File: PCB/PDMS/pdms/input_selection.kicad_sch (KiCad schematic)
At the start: 31 parts, among them U1 AQY221R4VY, U4 AQY221R4VY, U5 AQY221R4VY, U6 AQY221R4VY

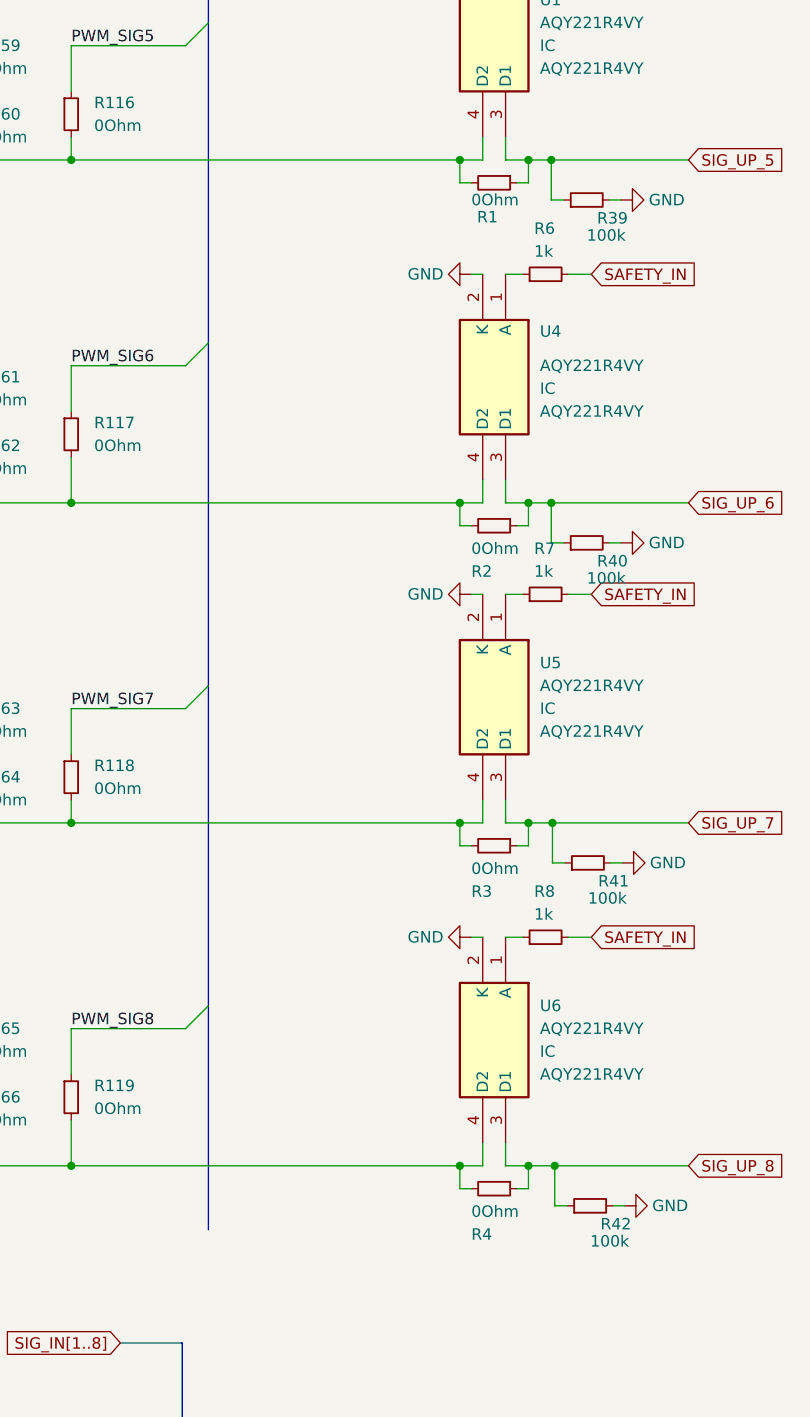
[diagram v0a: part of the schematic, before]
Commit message: Minor changes in overall schematics & MP4322 scheamtics
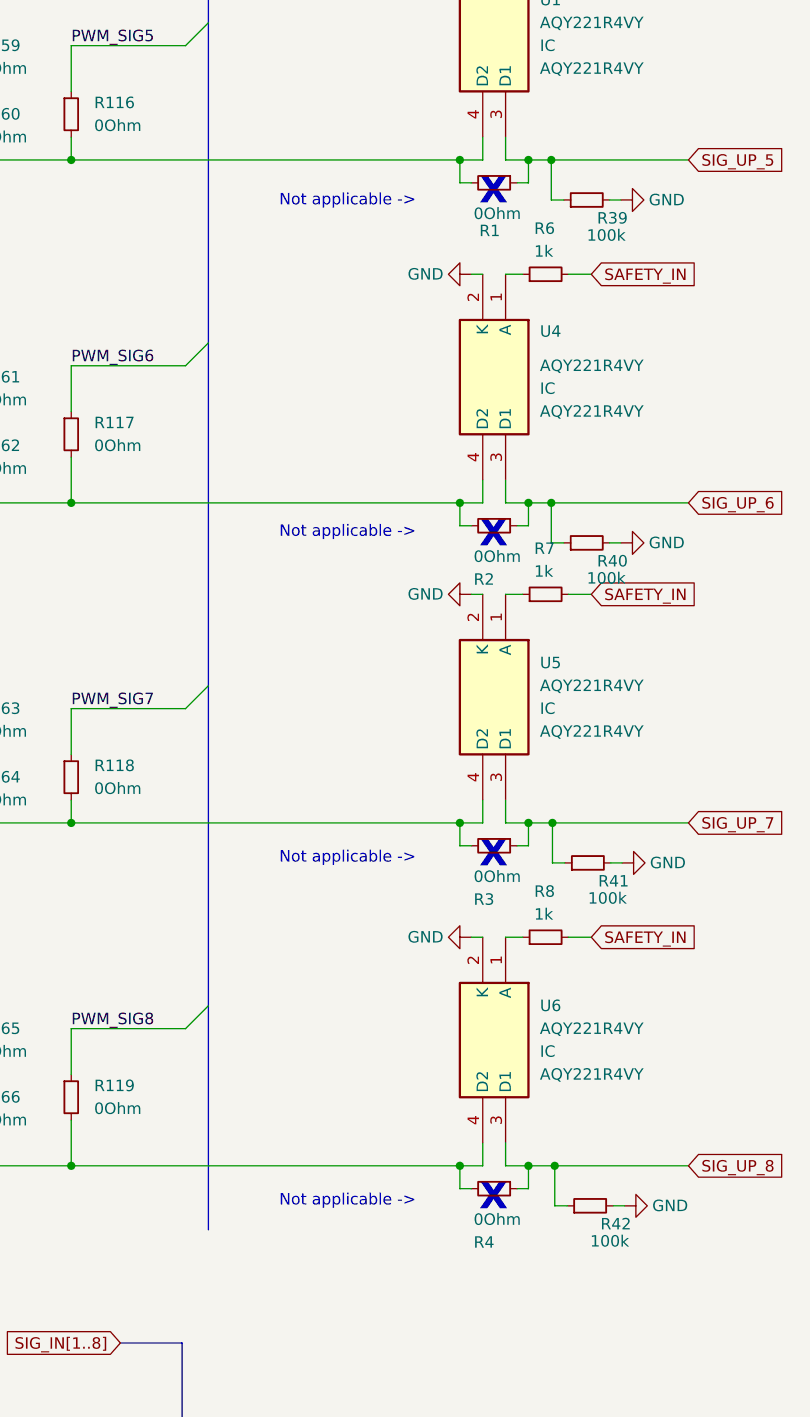
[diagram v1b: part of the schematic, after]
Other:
- note added: "Not applicable ->"
- note added: "X"
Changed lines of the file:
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@@
     (effects (font (size 2 2)) (justify left bottom))
+  )
+  (text "Not applicable ->" (at 114.935 136.525 0)
+    (effects (font (size 1.27 1.27)) (justify left bottom))
+  )
+  (text "Not applicable ->" (at 114.935 174.625 0)
+    (effects (font (size 1.27 1.27)) (justify left bottom))
   )
   (text "Safety section (safety line handler)" (at 99.568 277.876 0)
     (effects (font (size 2 2) italic) (justify left bottom))
   )
+  (text "X" (at 137.16 137.16 0)
+    (effects (font (size 3 3) (thickness 0.6) bold) (justify left bottom))
+  )
+  (text "X" (at 137.16 101.6 0)
+    (effects (font (size 3 3) (thickness 0.6) bold) (justify left bottom))
+  )
+  (text "Not applicable ->" (at 114.935 100.33 0)
+    (effects (font (size 1.27 1.27)) (justify left bottom))
+  )
   (text "Resistance should be selected for correct safety line voltage"
     (at 34.544 16.637 0)
@@
     (at 34.544 25.527 0)
     (effects (font (size 1.27 1.27)) (justify left bottom))
+  )
+  (text "X" (at 137.16 63.5 0)
+    (effects (font (size 3 3) (thickness 0.6) bold) (justify left bottom))
+  )
+  (text "Not applicable ->" (at 114.935 63.5 0)
+    (effects (font (size 1.27 1.27)) (justify left bottom))
+  )
+  (text "X" (at 137.16 175.26 0)
+    (effects (font (size 3 3) (thickness 0.6) bold) (justify left bottom))
   )
   (text "TODO Rev 3.0:\nAdd pull-down to all 16-channels input"
@@
   )
   (symbol (lib_id "Device:R_Small") (at 138.811 60.706 270) (unit 1)
-    (in_bom yes) (on_board yes) (fields_autoplaced)
-    (property "Reference" "R1" (id 0) (at 136.906 64.516 90)
-      (effects (font (size 1.27 1.27)) (justify left))
-    )
-    (property "Value" "0Ohm" (id 1) (at 136.271 62.611 90)
+    (in_bom yes) (on_board yes)
+    (property "Reference" "R1" (id 0) (at 137.16 66.04 90)
+      (effects (font (size 1.27 1.27)) (justify left))
+    )
+    (property "Value" "0Ohm" (id 1) (at 136.525 64.135 90)
       (effects (font (size 1.27 1.27)) (justify left))
     )
@@
   )
   (symbol (lib_id "Device:R_Small") (at 138.811 98.806 270) (unit 1)
-    (in_bom yes) (on_board yes) (fields_autoplaced)
-    (property "Reference" "R2" (id 0) (at 136.271 103.886 90)
-      (effects (font (size 1.27 1.27)) (justify left))
-    )
-    (property "Value" "0Ohm" (id 1) (at 136.271 101.346 90)
+    (in_bom yes) (on_board yes)
+    (property "Reference" "R2" (id 0) (at 136.525 104.775 90)
+      (effects (font (size 1.27 1.27)) (justify left))
+    )
+    (property "Value" "0Ohm" (id 1) (at 136.525 102.235 90)
       (effects (font (size 1.27 1.27)) (justify left))
     )
@@
   )
   (symbol (lib_id "Device:R_Small") (at 138.811 134.366 270) (unit 1)
-    (in_bom yes) (on_board yes) (fields_autoplaced)
-    (property "Reference" "R3" (id 0) (at 136.271 139.446 90)
-      (effects (font (size 1.27 1.27)) (justify left))
-    )
-    (property "Value" "0Ohm" (id 1) (at 136.271 136.906 90)
+    (in_bom yes) (on_board yes)
+    (property "Reference" "R3" (id 0) (at 136.525 140.335 90)
+      (effects (font (size 1.27 1.27)) (justify left))
+    )
+    (property "Value" "0Ohm" (id 1) (at 136.525 137.795 90)
       (effects (font (size 1.27 1.27)) (justify left))
     )
@@
   )
   (symbol (lib_id "Device:R_Small") (at 138.811 172.466 270) (unit 1)
-    (in_bom yes) (on_board yes) (fields_autoplaced)
-    (property "Reference" "R4" (id 0) (at 136.271 177.546 90)
-      (effects (font (size 1.27 1.27)) (justify left))
-    )
-    (property "Value" "0Ohm" (id 1) (at 136.271 175.006 90)
-      (effects (font (size 1.27 1.27)) (justify left))
-    )
+    (in_bom yes) (on_board yes)
+    (property "Reference" "R4" (id 0) (at 136.525 178.435 90)
+      (effects (font (size 1.27 1.27)) (justify left))
+    )
+    (property "Value" "0Ohm" (id 1) (at 136.525 175.895 90)
+      (effects (font (size 1.27 1.27)) (justify left))
+    )
